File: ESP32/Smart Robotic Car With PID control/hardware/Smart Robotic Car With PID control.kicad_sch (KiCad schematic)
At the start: 0 parts

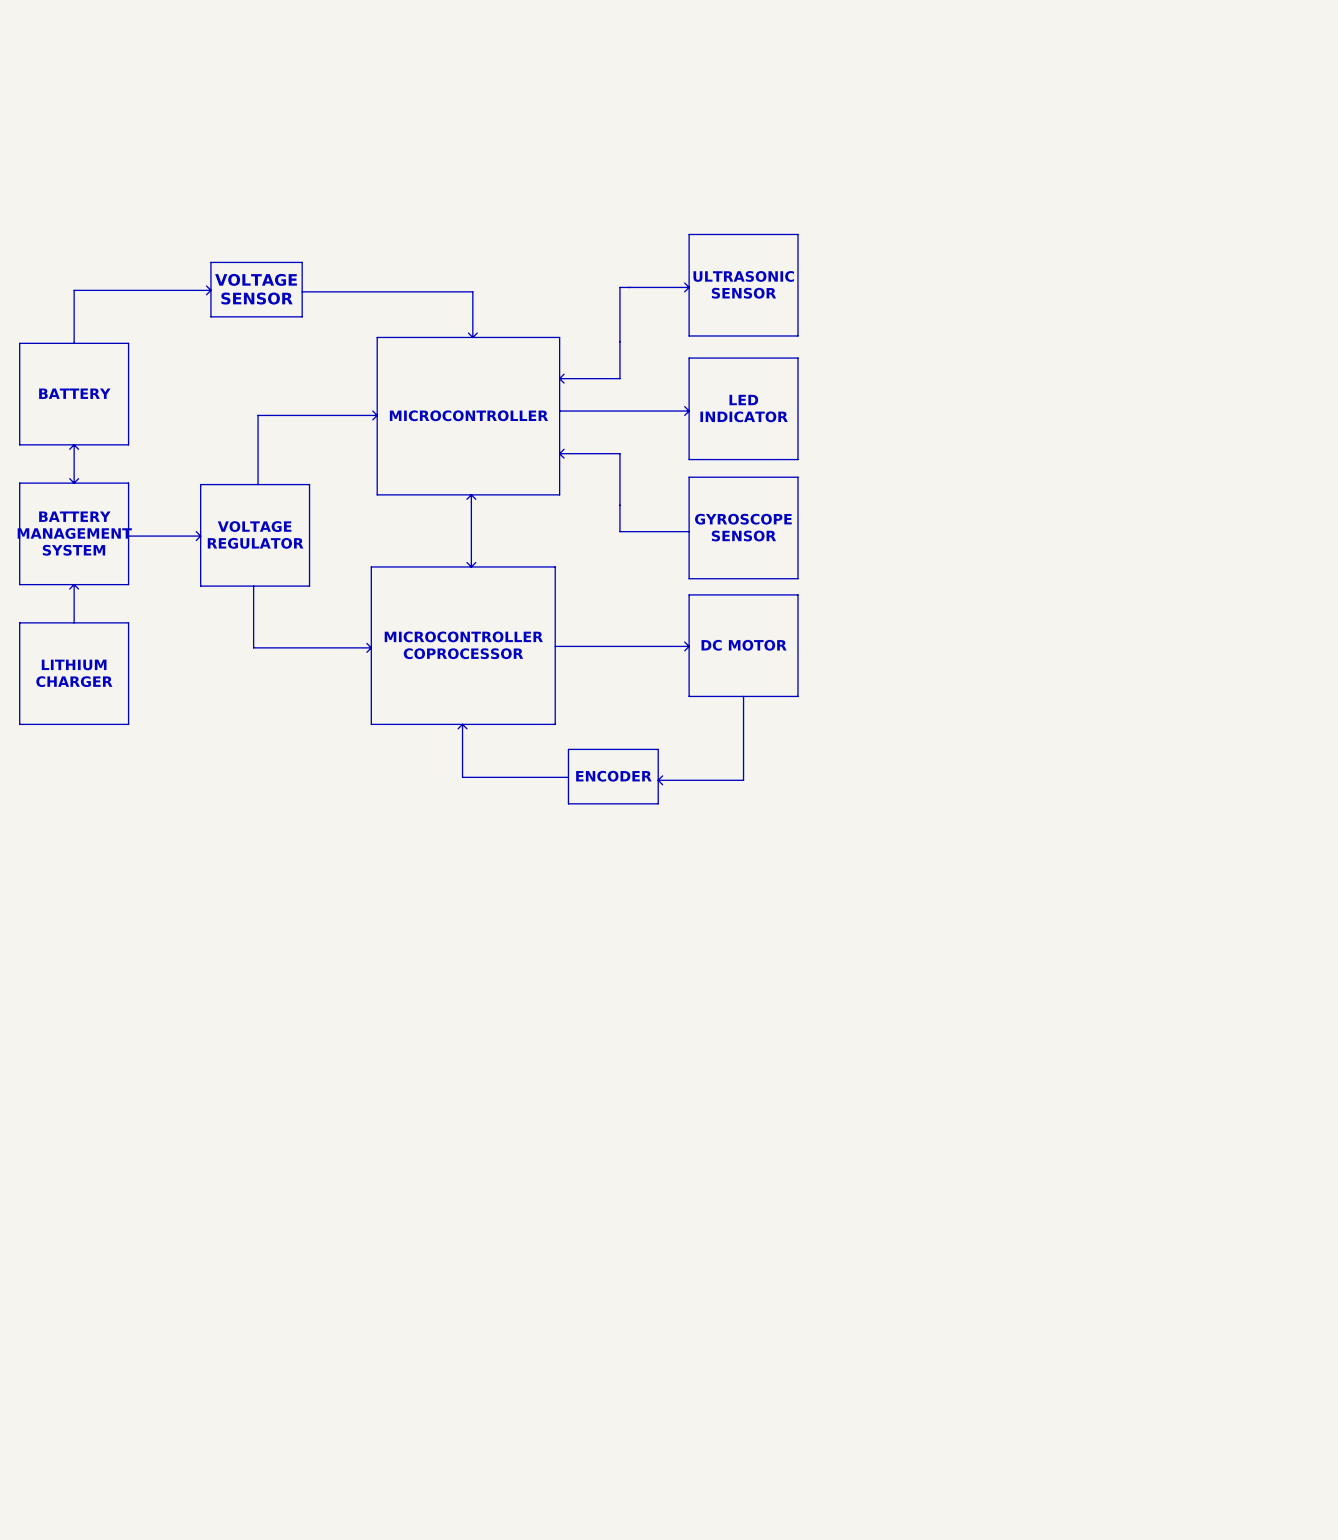
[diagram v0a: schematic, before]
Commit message: Update from work
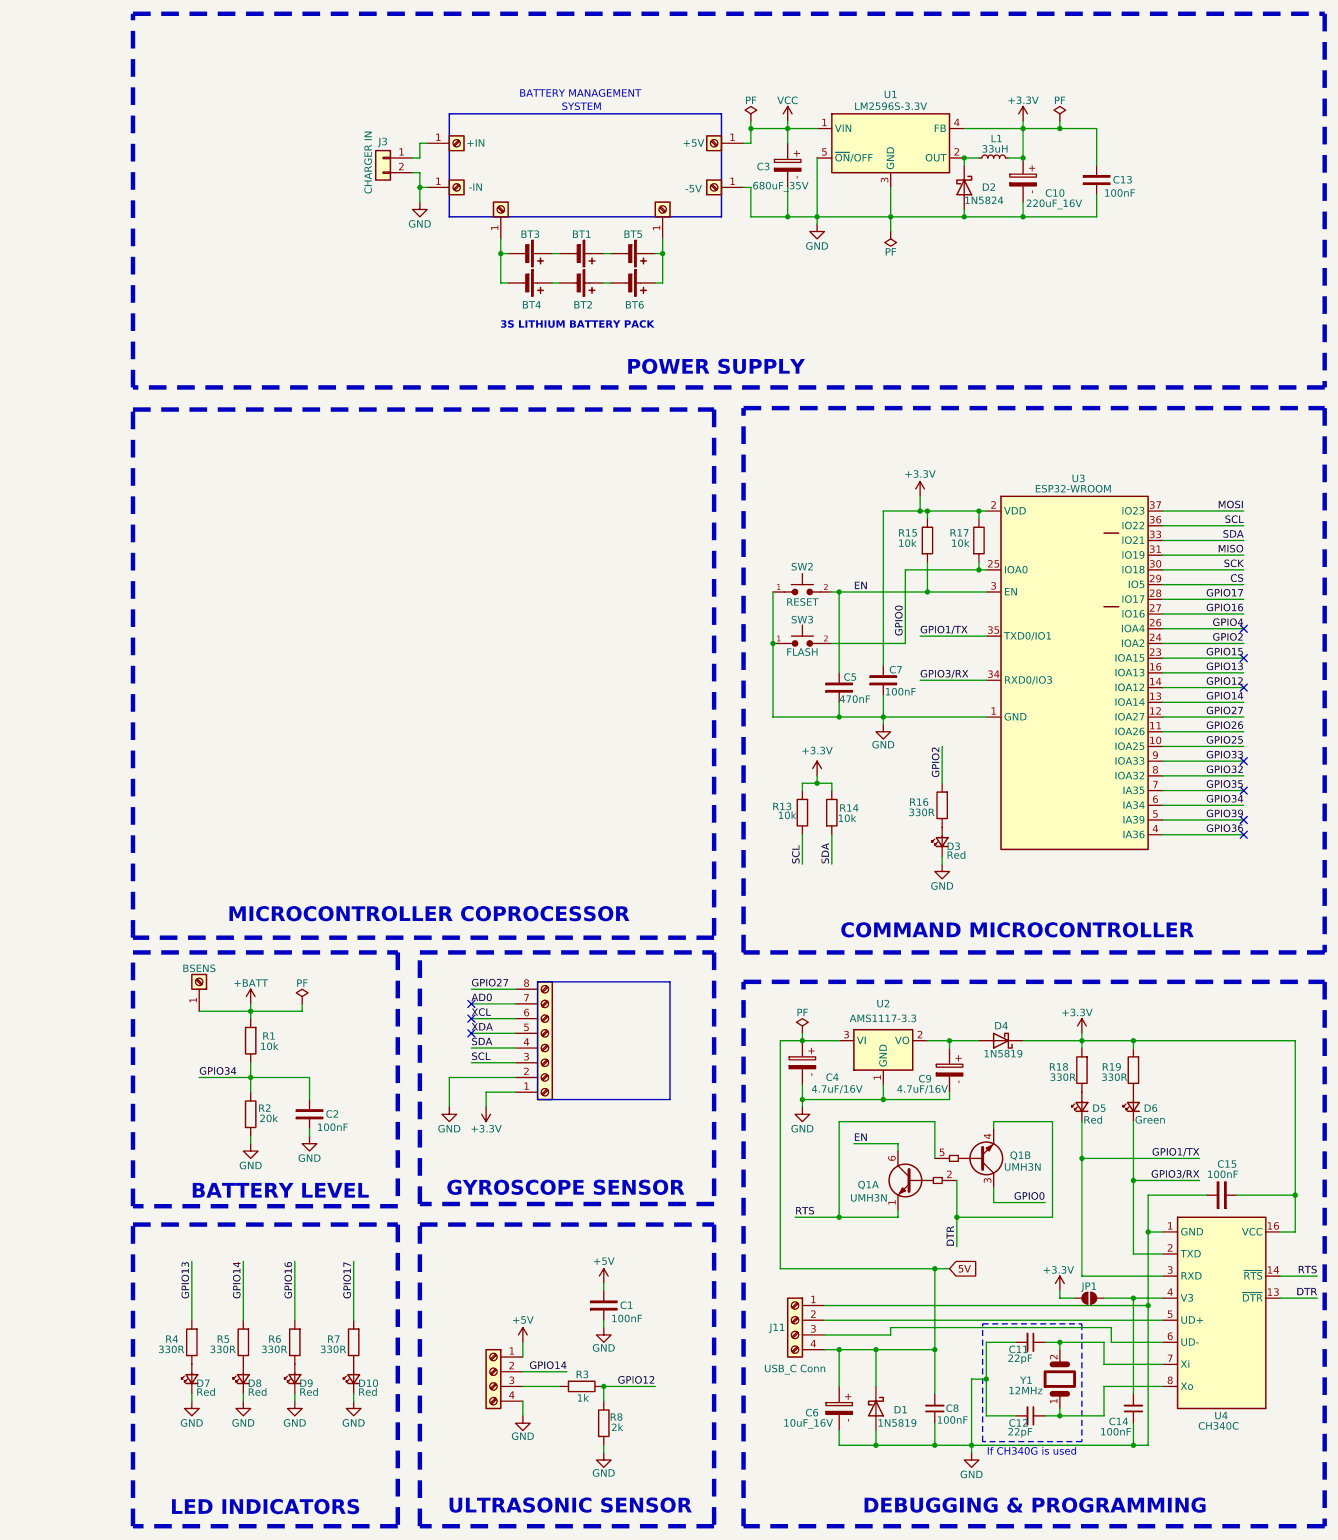
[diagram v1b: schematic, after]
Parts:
- added BT1, BT2, BT3, BT4, BT5, BT6: Battery_Cell, symbol Device:Battery_Cell
- added C1, C13, C15, C2, C7: 100nF, Capacitor_SMD:C_0805_2012Metric_Pad1.18x1.45mm_HandSolder, symbol PCM_SL_Capacitors:104_Ceramic
- added C10: 220uF_16V, Capacitor_SMD:CP_Elec_6.3x7.7, symbol PCM_SL_Capacitors:470uF_35V
- added C11, C12: 22pF, Capacitor_SMD:C_0805_2012Metric_Pad1.18x1.45mm_HandSolder, symbol Device:C_Small
- added C14, C8: 100nF, Capacitor_SMD:C_0805_2012Metric_Pad1.18x1.45mm_HandSolder, symbol Device:C_Small
- added C3: 680uF_35V, Capacitor_SMD:CP_Elec_10x12.5, symbol PCM_SL_Capacitors:470uF_35V
- added C4, C9: 4.7uF/16V, Capacitor_Tantalum_SMD:CP_EIA-3528-21_Kemet-B_HandSolder, symbol PCM_SL_Capacitors:4.7uF_16V
- added C5: 470nF, Capacitor_SMD:C_0805_2012Metric_Pad1.18x1.45mm_HandSolder, symbol PCM_SL_Capacitors:104_Ceramic
- added C6: 10uF_16V, Capacitor_THT:CP_Radial_D5.0mm_P2.00mm, symbol PCM_SL_Capacitors:10uF_16V
- added D1, D4: 1N5819, Diode_SMD:D_SMA, symbol Diode:1N5819
- added D10, D3, D5, D7, D8, D9: Red, LED_THT:LED_D3.0mm, symbol SparkFun-LED:LED_Red_0603
- added D2: 1N5824, Diode_SMD:D_SMA, symbol Diode:1N5822
- added D6: Green, LED_THT:LED_D3.0mm, symbol SparkFun-LED:LED_Red_0603
- added J1: MPU6050, symbol Connector:Screw_Terminal_01x08
- added J10: -5V, TestPoint:TestPoint_Keystone_5015_Micro_Mini, symbol Connector:Screw_Terminal_01x01
- added J11: USB_C Conn, Connector_PinHeader_2.54mm:PinHeader_1x04_P2.54mm_Vertical, symbol Connector:Screw_Terminal_01x04
- added J2: Ultra Sonic, Connector_PinSocket_2.54mm:PinSocket_1x04_P2.54mm_Vertical, symbol Connector:Screw_Terminal_01x04
- added J24: BSENS, Connector_Wire:SolderWire-0.1sqmm_1x01_D0.4mm_OD1mm, symbol Connector:Screw_Terminal_01x01
- added J3: CHARGER IN, symbol Connector_Generic:Conn_01x02
- added J5: +IN, TestPoint:TestPoint_Keystone_5015_Micro_Mini, symbol Connector:Screw_Terminal_01x01
- added J6: -IN, TestPoint:TestPoint_Keystone_5015_Micro_Mini, symbol Connector:Screw_Terminal_01x01
- added J7: -BATT, symbol Connector:Screw_Terminal_01x01
- added J8: +BATT, symbol Connector:Screw_Terminal_01x01
- added J9: +5V, TestPoint:TestPoint_Keystone_5015_Micro_Mini, symbol Connector:Screw_Terminal_01x01
- added JP1: ~, Jumper:SolderJumper-2_P1.3mm_Open_Pad1.0x1.5mm, symbol SparkFun-Jumper:SolderJumper_2_Open
- added L1: 33uH, Inductor_SMD:L_12x12mm_H6mm, symbol Device:L_Small
- added Q1: UMH3N, Package_TO_SOT_SMD:SOT-363_SC-70-6, symbol Transistor_BJT:UMH3N
- added R1, R13, R14, R15, R17: 10k, Resistor_SMD:R_0805_2012Metric, symbol PCM_SL_Resistors:10k
- added R16, R18, R19, R4, R5, R6, R7: 330R, Resistor_SMD:R_0805_2012Metric, symbol PCM_SL_Resistors:1M
- added R2: 20k, Resistor_SMD:R_0805_2012Metric, symbol PCM_SL_Resistors:10k
- added R3: 1k, Resistor_SMD:R_0805_2012Metric, symbol PCM_SL_Resistors:10k
- added R8: 2k, Resistor_SMD:R_0805_2012Metric, symbol PCM_SL_Resistors:10k
- added SW2: RESET, Button_Switch_SMD:SW_SPST_CK_KXT3, symbol PCM_SL_Devices:Push_Button
- added SW3: FLASH, Button_Switch_SMD:SW_SPST_CK_KXT3, symbol PCM_SL_Devices:Push_Button
- added U1: LM2596S-3.3V, Package_TO_SOT_SMD:TO-263-5_TabPin6, symbol Regulator_Switching:LM2596S-3.3
- added U2: AMS1117-3.3, Package_TO_SOT_SMD:SOT-223-3_TabPin2, symbol Regulator_Linear:AMS1117-3.3
- added U3: ESP32-WROOM, RF_Module:ESP32-WROOM-32U, symbol SparkFun-RF:ESP32-WROOM
- added U4: CH340C, Package_SO:SOIC-16_3.9x9.9mm_P1.27mm, symbol Interface_USB:CH340C
- added Y1: 12MHz, Crystal:Crystal_HC49-4H_Vertical, symbol PCM_SL_Devices:Crystal_16MHz
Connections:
- new net: C14.2, JP1.1 (A), U4.4 (V3)
- new net: J11.2 (Pin_2), U4.5 (UD+)
- new net: J11.3 (Pin_3), U4.6 (UD-)
- new net: C11.1, U4.7 (Xi), Y1.2
- new net: C12.1, U4.8 (Xo), Y1.1
- new net: D5.2 (A), R18.2
- new net: BT1.2 (-), BT3.1 (+)
- new net: BT3.2 (-), BT4.2 (-), J7.1 (Pin_1)
- new net: D9.2 (A), R6.2
- new net: BT5.1 (+), BT6.1 (+), J8.1 (Pin_1)
- new net: BT1.1 (+), BT5.2 (-)
- new net: C9.1, D4.2 (A), U2.2 (VO)
- new net: D3.2 (A), R16.2
- new net: D8.2 (A), R5.2
- new net: D2.1 (K), L1.1, U1.2 (OUT)
- new net: J3.1 (Pin_1), J5.1 (Pin_1)
- new net: J2.3 (Pin_3), R3.1
- new net: D7.2 (A), R4.2
- new net: BT2.2 (-), BT4.1 (+)
- new net: BT2.1 (+), BT6.2 (-)
- new net: D10.2 (A), R7.2
- new net: D6.2 (A), R19.2
- new net +3.3V: C10.1, C13.2, C15.1, C7.2, D4.1 (K), J1.1 (Pin_1), JP1.2 (B), L1.2, R13.1, R14.2, R15.2, R17.2, R18.1, R19.1, U1.4 (FB), U3.2 (VDD), U4.16 (VCC)
- new net +5V: C1.2, J2.1 (Pin_1)
- new net +BATT: J24.1 (Pin_1), R1.1
- new net 5V: C4.1, C6.1, C8.2, D1.1 (K), J11.4 (Pin_4), U2.3 (VI)
- new net AD0: J1.7 (Pin_7)
- new net CS: U3.29 (IO5)
- new net DTR: Q1.2 (B1), Q1.4 (E2), U4.13 (~{DTR})
- new net EN: C5.2, Q1.6 (C1), R15.1, SW2.2, U3.3 (EN)
- new net GND: C1.1, C10.2, C11.2, C12.2, C13.1, C14.1, C15.2, C2.1, C3.2, C4.2, C5.1, C6.2, C7.1, C8.1, C9.2, D1.2 (A), D10.1 (K), D2.2 (A), D3.1 (K), D7.1 (K), D8.1 (K), D9.1 (K), J1.2 (Pin_2), J10.1 (Pin_1), J11.1 (Pin_1), J2.4 (Pin_4), J3.2 (Pin_2), J6.1 (Pin_1), R2.1, R8.1, SW2.1, SW3.1, U1.3 (GND), U1.5 (~{ON}/OFF), U1.6 (GND), U2.1 (GND), U3.1 (GND), U3.15 (GND), U3.38 (GND), U3.39 (GND), U4.1 (GND)
- new net GPIO0: Q1.3 (C2), R17.1, SW3.2, U3.25 (IOA0)
- new net GPIO12: R3.2, R8.2, U3.14 (IOA12)
- new net GPIO13: R4.1, U3.16 (IOA13)
- new net GPIO14: J2.2 (Pin_2), R5.1, U3.13 (IOA14)
- new net GPIO15: U3.23 (IOA15)
- new net GPIO16: R6.1, U3.27 (IO16)
- new net GPIO17: R7.1, U3.28 (IO17)
- new net GPIO1/TX: D5.1 (K), U3.35 (TXD0/IO1), U4.3 (RXD)
- new net GPIO2: R16.1, U3.24 (IOA2)
- new net GPIO25: U3.10 (IOA25)
- new net GPIO26: U3.11 (IOA26)
- new net GPIO27: J1.8 (Pin_8), U3.12 (IOA27)
- new net GPIO32: U3.8 (IOA32)
- new net GPIO33: U3.9 (IOA33)
- new net GPIO34: C2.2, R1.2, R2.2, U3.6 (IA34)
- new net GPIO35: U3.7 (IA35)
- new net GPIO36: U3.4 (IA36)
- new net GPIO39: U3.5 (IA39)
- new net GPIO3/RX: D6.1 (K), U3.34 (RXD0/IO3), U4.2 (TXD)
- new net GPIO4: U3.26 (IOA4)
- new net MISO: U3.31 (IO19)
- new net MOSI: U3.37 (IO23)
- new net RTS: Q1.1 (E1), Q1.5 (B2), U4.14 (~{RTS})
- new net SCK: U3.30 (IO18)
- new net SCL: J1.3 (Pin_3), R13.2, U3.36 (IO22)
- new net SDA: J1.4 (Pin_4), R14.1, U3.33 (IO21)
- new net VCC: C3.1, J9.1 (Pin_1), U1.1 (VIN)
- new net XCL: J1.6 (Pin_6)
- new net XDA: J1.5 (Pin_5)
- no-connect marks 0 -> 10
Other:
- note added: "3S LITHIUM BATTERY PACK"
- note added: "BATTERY LEVEL"
- note added: "BATTERY MANAGEMENT"
- note added: "COMMAND MICROCONTROLLER"
- note added: "DEBUGGING & PROGRAMMING"
- note added: "GYROSCOPE SENSOR"
- note added: "If CH340G is used"
- note added: "LED INDICATORS"
- note added: "MICROCONTROLLER COPROCESSOR"
- note added: "POWER SUPPLY"
- note added: "SYSTEM"
- note added: "ULTRASONIC SENSOR"
